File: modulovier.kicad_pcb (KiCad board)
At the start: 2 copper layers, 19 parts, among them J1 EXT. PORT, J2 oled, J3 leds, SW1 mx, SW2 mx, SW3 mx, SW4 mx, SW5 volume, U2 Pico

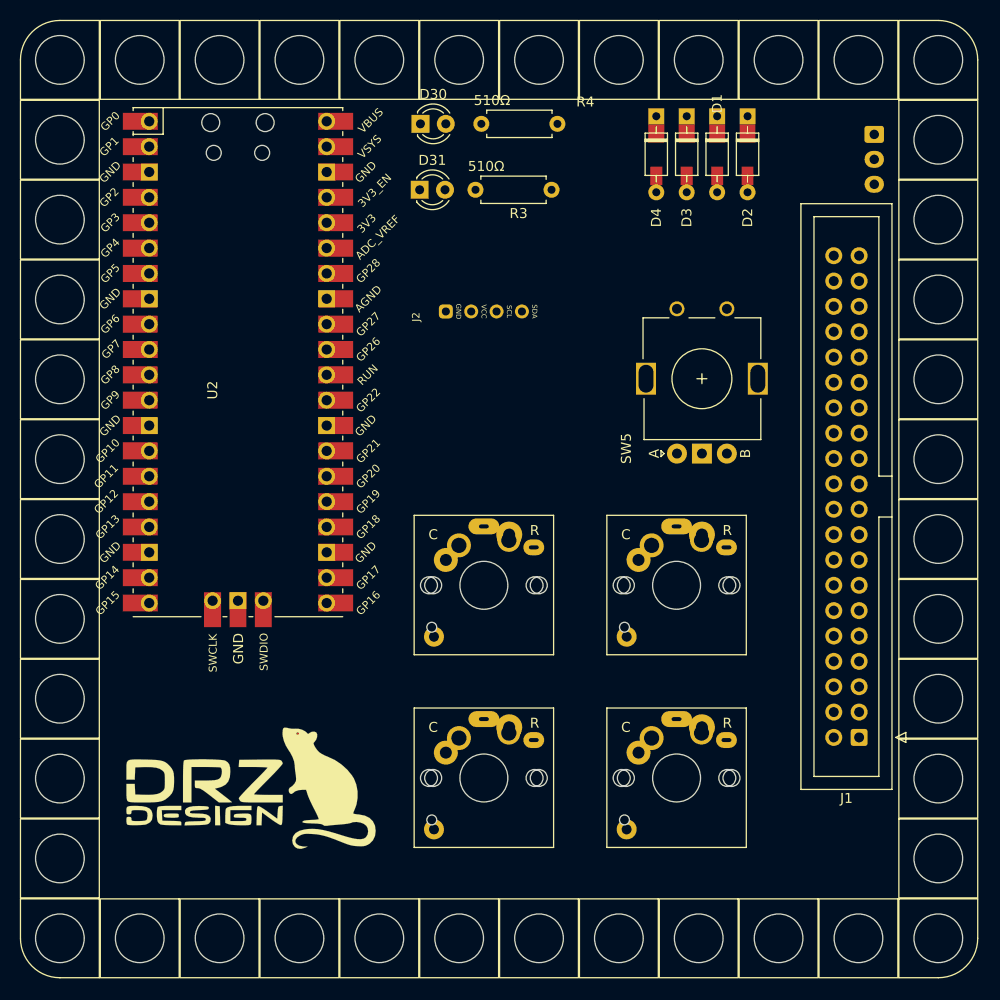
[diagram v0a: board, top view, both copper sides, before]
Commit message: Finished work to verify
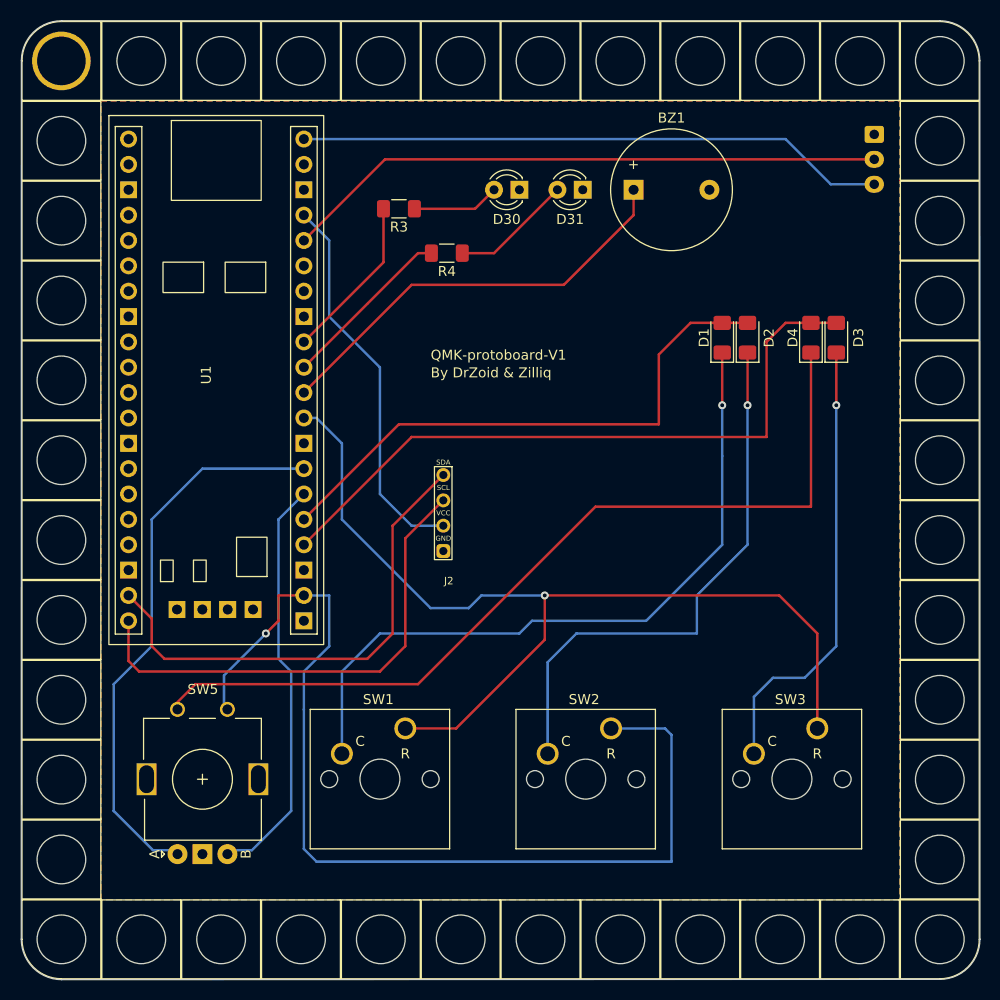
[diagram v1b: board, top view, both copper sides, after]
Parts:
- removed G***: LOGO, drz:LOGO_DRZ_DESIGN
- removed J1: EXT. PORT, Connector_IDC:IDC-Header_2x20_P2.54mm_Vertical
- removed SW4: mx, m-lego:CherryMX_ChocV2_1u
- removed U2: Pico, m-lego:RPi_Pico_SMD_TH
- added BZ1: Buzzer, Buzzer_Beeper:Buzzer_12x9.5RM7.6, F.Cu at (115.6, 38.1)
- added U1: WeAct-RP2040-Pico, WeAct RP2040:WeAct-RP2040-Pico, F.Cu at (73.8, 57.2)
- D1, D2, D3, D4: footprint m65:diode_v -> Diode_SMD:D_1206_3216Metric_Pad1.42x1.75mm_HandSolder
- D30: footprint m65:LED_D3.0mm_lwr -> M65Lego:LED_D3.0mm_lwr
- D31: footprint m65:LED_D3.0mm_rse -> M65Lego:LED_D3.0mm_rse
- H1: footprint m-lego:LegoHole_12x12u_4875 -> M65Lego:LegoHole_12x12u_4875
- J2: footprint m-lego:OLED_128x32 -> M65Lego:OLED_128x32
- R3, R4: footprint m65:R510_led -> Resistor_SMD:R_1206_3216Metric_Pad1.30x1.75mm_HandSolder
- SW1, SW2, SW3: footprint m-lego:CherryMX_ChocV2_1u-3dchocov2 -> M65Lego:SW_Cherry_MX_1.00u_PCB
- SW5: footprint m65:RotaryEncoder_Alps_EC11E_Vertical_H20mm -> M65Lego:RotaryEncoder_Alps_EC11E_Vertical_H20mm
- moved SW5 57.7 mm to (72.4, 97.2)
- moved SW3 36.5 mm to (131.4, 97.1)
- moved D4 27.1 mm to (133.3, 52.9), turned to 90 degrees
- moved D3 26.8 mm to (135.9, 52.9), turned to 90 degrees
- moved D1 22.2 mm to (124.5, 52.9), turned to 90 degrees
- moved D2 22.2 mm to (127.0, 52.9), turned to 90 degrees
- moved J2 20.6 mm to (96.5, 70.5), turned to -90 degrees
- moved R4 17.0 mm to (96.9, 44.5)
- moved D31 16.3 mm to (110.5, 38.1), turned to 180 degrees
- moved R3 15.4 mm to (92.1, 40.0)
- moved D30 11.9 mm to (104.1, 38.1), turned to 180 degrees
- moved SW1 10.4 mm to (90.2, 97.1)
- moved SW2 9.10 mm to (110.8, 97.1)
- moved H1 0.18 mm to (58.3, 25.2)
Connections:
- D4 pad 1: Net-(D4-Pad1) -> Net-(D4-K)
- SW5 pad C: gnd -> GND
- SW5 pad S1: Net-(D5-Pad1) -> Net-(D4-K)
- SW5 pad S2: r1 -> r2
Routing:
- net r2: track 0.00 -> 101.2 mm, vias 0 -> 1
- net r1: track 0.00 -> 97.5 mm, vias 0 -> 1
- net Net-(D4-K): track 0.00 -> 87.5 mm
- net Net-(D1-K): track 0.00 -> 70.9 mm, vias 0 -> 1
- net c2: track 0.00 -> 68.1 mm
- net leds_data: track 0.00 -> 60.5 mm
- net 5V: track 0.00 -> 59.0 mm
- net c1: track 0.00 -> 56.7 mm
- net ea: track 0.00 -> 55.8 mm
- net Net-(D2-K): track 0.00 -> 55.6 mm, vias 0 -> 1
- net SDA: track 0.00 -> 49.7 mm
- net SCL: track 0.00 -> 49.4 mm
- net Net-(D3-K): track 0.00 -> 45.5 mm, vias 0 -> 1
- net buz: track 0.00 -> 42.9 mm
- net eb: track 0.00 -> 41.7 mm
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- added copper zone on B.Cu, net GND
- added copper zone on F.Cu, net GND
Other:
- board outline added: 96 x 96.1 mm
- board text added: "By DrZoid & Zilliq"
- board text added: "QMK-protoboard-V1"
